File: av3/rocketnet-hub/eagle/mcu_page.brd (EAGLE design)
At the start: 113 x 77 mm, 333 parts, among them J1 ROCKETBUS, J2 ROCKETBUS, J3 ROCKETBUS, J4 ROCKETBUS, J5 ROCKETBUS, J6 ROCKETBUS, J7 ROCKETBUS, J8 ROCKETBUS, Q1 25.000MHz, X1 87758-0416, X2 87758-0416, X3 87758-0416, X4 87758-0416, X5 87758-0416, X6 87758-0416, X7 87758-0416, X8 87758-0416

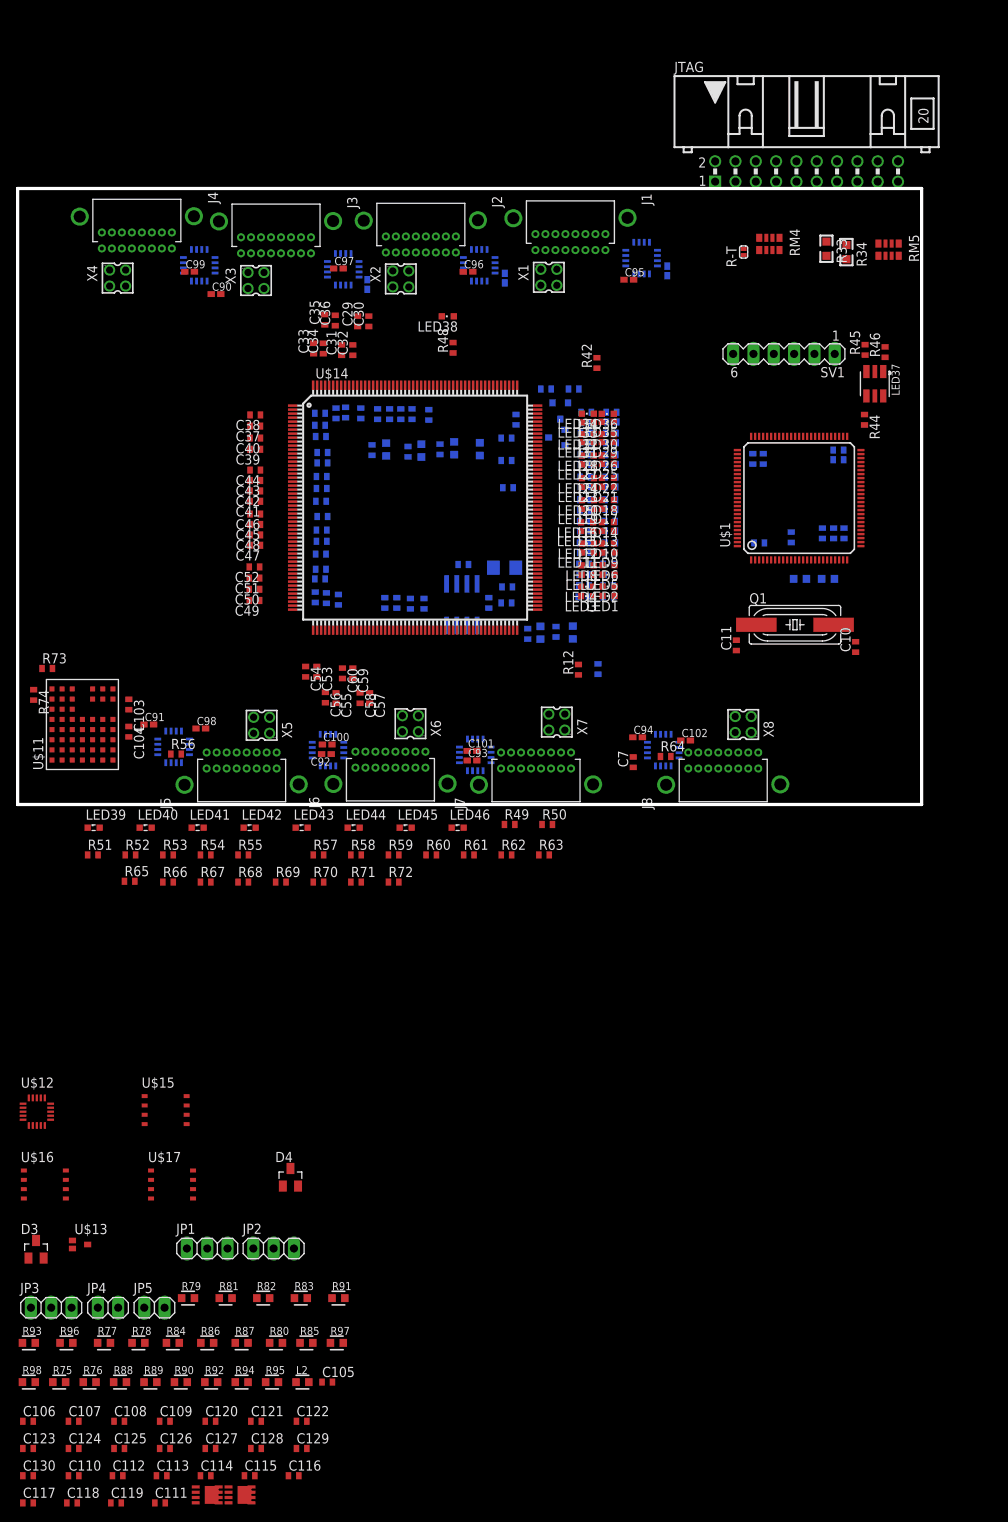
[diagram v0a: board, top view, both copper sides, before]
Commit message: layout updates
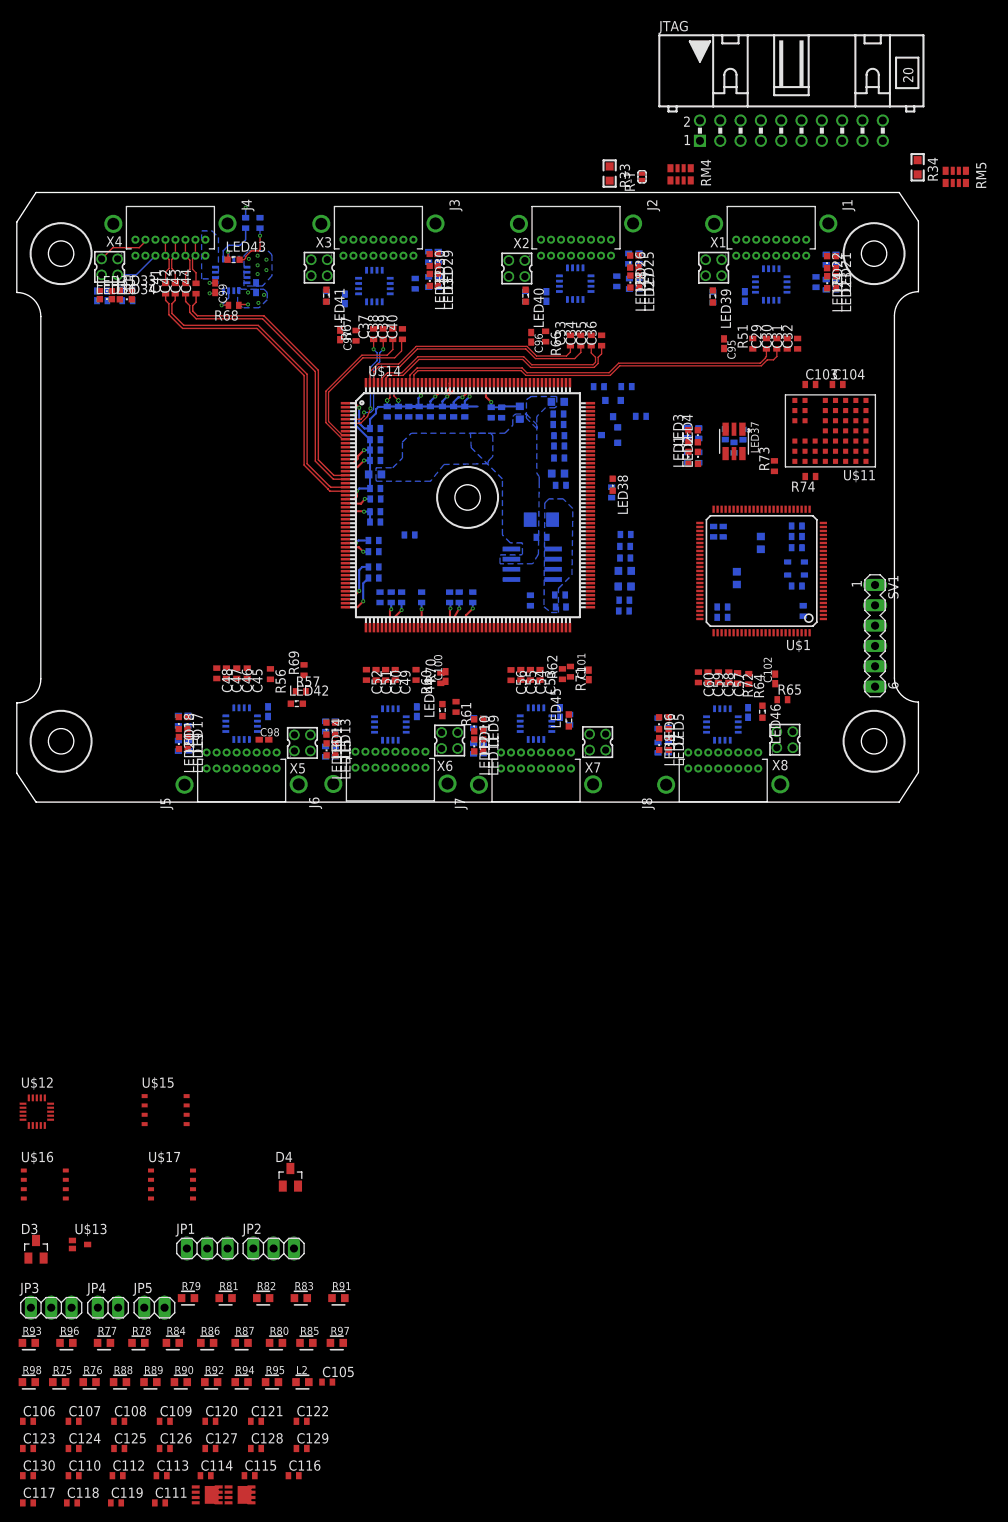
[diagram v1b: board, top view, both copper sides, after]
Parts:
- removed C10, C11: 27p, rcl:C0402
- removed Q1: 25.000MHz, crystal:SM49
- added U$20: ASE, crystal:ASE
- added U$21, U$22, U$23, U$24, U$25: #4-BARE_MOUNTING_HOLE/.300, mount:#4/.300-BARE+STD_NUT_OR_STAR_WASHER
- moved R51 104.4 mm to (96.9, 72.6), turned to 90 degrees
- moved LED39 102.0 mm to (91.9, 78.5), turned to 270 degrees
- moved R74 100.9 mm to (104.1, 56.0), turned to 180 degrees
- moved U$11 100.4 mm to (106.6, 61.7), turned to 180 degrees
- moved C104 98.7 mm to (107.5, 67.5), turned to 0 degrees
- moved R73 94.4 mm to (99.6, 57.3), turned to 90 degrees
- moved C103 94.1 mm to (104.1, 67.5), turned to 0 degrees
- moved R52 94.0 mm to (79.9, 80.4), flipped to the bottom, turned to 90 degrees
- moved R65 84.7 mm to (100.6, 28.1)
- moved R66 82.9 mm to (71.0, 73.5), turned to 270 degrees
- moved R53 82.9 mm to (68.5, 78.5), flipped to the bottom, turned to 90 degrees
- moved LED40 81.7 mm to (68.5, 78.6), turned to 270 degrees
- moved R59 80.7 mm to (35.3, 87.7), flipped to the bottom, turned to 90 degrees
- moved R58 80.2 mm to (33.5, 87.7), flipped to the bottom, turned to 270 degrees
- moved R49 77.9 mm to (104.8, 80.3), flipped to the bottom, turned to 90 degrees
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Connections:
- net N$23 renamed RX1_N
- net N$24 renamed RX2_N
- net N$25 renamed TX1_P
- net N$26 renamed TX2_P
- net N$29 renamed RX3_N
- net N$30 renamed TX3_P
- net N$31 renamed RX4_N
- net N$32 renamed TX4_P
- net NODE2_RXM renamed NODE2_RX_N
- net NODE2_RXP renamed NODE2_RX_P
- net NODE2_TXM renamed NODE2_TX_N
- net NODE3_RXM renamed NODE3_RX_N
- net NODE3_RXP renamed NODE3_RX_P
- net NODE3_TXM renamed NODE3_TX_N
- net NODE3_TXP renamed NODE3_TX_P
- net NODE4_RXM renamed NODE4_RX_N
- net NODE4_RXP renamed NODE4_RX_P
- net NODE4_TXM renamed NODE4_TX_N
- net NODE4_TXP renamed NODE4_TX_P
- net RXP1 renamed RX1_P
- net RXP2 renamed RX2_P
- net RXP3 renamed RX3_P
- net RXP4 renamed RX4_P
- net TXM1 renamed TX1_N
- net TXM2 renamed TX2_N
- net TXM3 renamed TX3_N
- net TXM4 renamed TX4_N
- removed net N$125: C90.2, U$6.5
- removed net N$152: R71.2
- removed net N$153: R72.2
- removed net N$154: U$7.8
- removed net N$155: U$9.8
- removed net N$157: U$4.8
- removed net N$158: U$6.8
- removed net N$159: U$8.8
- removed net N$2 (its old number): C10.2, Q1.2, U$1.13
- removed net N$4 (its old number): C11.1
- removed net NODE1_ILIM: U$3.8
- removed net NODE8_ILIM: U$10.8
- new net N$130: R67.2, U$5.7
- new net NODE1_RX_N: C29.2
- new net NODE1_RX_P: C30.2
- new net NODE1_TX_P: C31.2, C32.2
- new net NODE2_TX_P: C36.2
- net +3V3: now also U$20.1, U$20.4
- net GND: now also C90.2, U$20.2, U$6.5; no longer C10.1
- net N$1: now also U$20.3; no longer C11.2, Q1.1
- net N$147: now also R68.2, U$6.7; no longer U$5.8
- net N$148: now also R69.2, U$7.7; no longer R67.2
- net N$149: now also R70.2, U$8.7; no longer R68.2
- net N$150: now also R71.2, U$9.7; no longer R69.2
- net N$151: now also R72.2, U$10.7; no longer R70.2
- net NODE1_RXM: no longer C29.2
- net NODE1_RXP: no longer C30.2
- net NODE1_TXM: no longer C31.2
- net NODE1_TXP: no longer C32.2
- net NODE2_TXP: no longer C36.2
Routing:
- net N$108: track 0.00 -> 111.3 mm, vias 0 -> 23
- net RX1_P: track 0.00 -> 48.8 mm
- net RX1_N: track 0.00 -> 48.0 mm
- net RX4_N: track 0.00 -> 40.6 mm
- net RX4_P: track 0.00 -> 39.9 mm
- net TX4_N: track 0.00 -> 37.2 mm
- net TX4_P: track 0.00 -> 36.5 mm
- net TX2_N: track 0.00 -> 31.2 mm
- net TX2_P: track 0.00 -> 31.1 mm
- net RX2_P: track 0.00 -> 30.1 mm
- net RX2_N: track 0.00 -> 29.2 mm
- net TX3_P: track 0.00 -> 19.3 mm
- net TX3_N: track 0.00 -> 19.1 mm
- net RX3_P: track 0.00 -> 13.5 mm, vias 0 -> 2
- net RX3_N: track 0.00 -> 13.3 mm, vias 0 -> 2
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- added copper zone on layer 15, net +18V
- added copper zone on layer 16, net +18V
- added copper zone on layer 16, net GND
- added copper zone on layer 2, net GND
- added copper zone on layer 16, net NODE4_VOUT
- added copper zone on layer 15, net TEMP
- added copper zone on layer 3, net TEMP
- added copper zone on layer 16, net VDD
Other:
- board size 113 x 77 mm -> 112.7 x 76.2 mm
